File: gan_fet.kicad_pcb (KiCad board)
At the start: 2 copper layers, 13 x 22.2 mm, 6 parts, among them J1 Conn_01x04_Male, Q1 EPC2036, U1 NPC81074

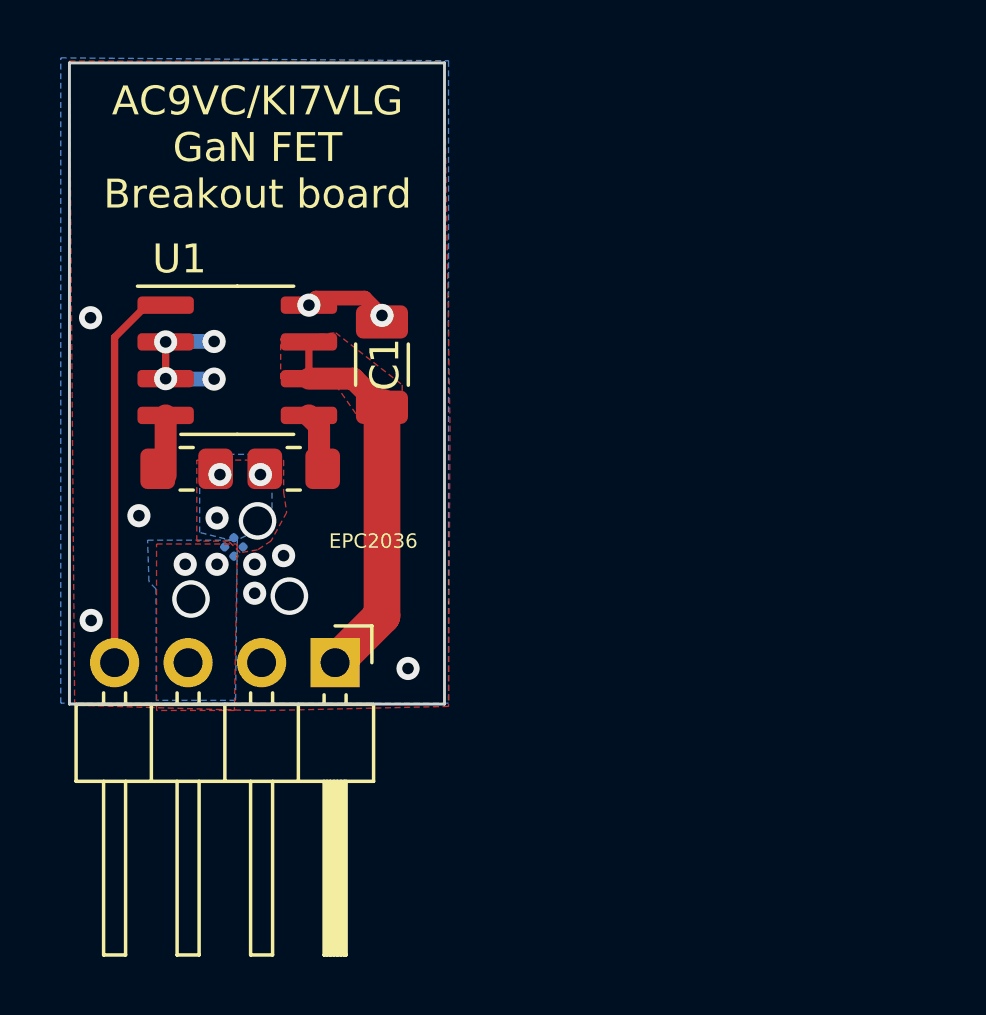
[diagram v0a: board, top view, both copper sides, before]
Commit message: rev_1 board
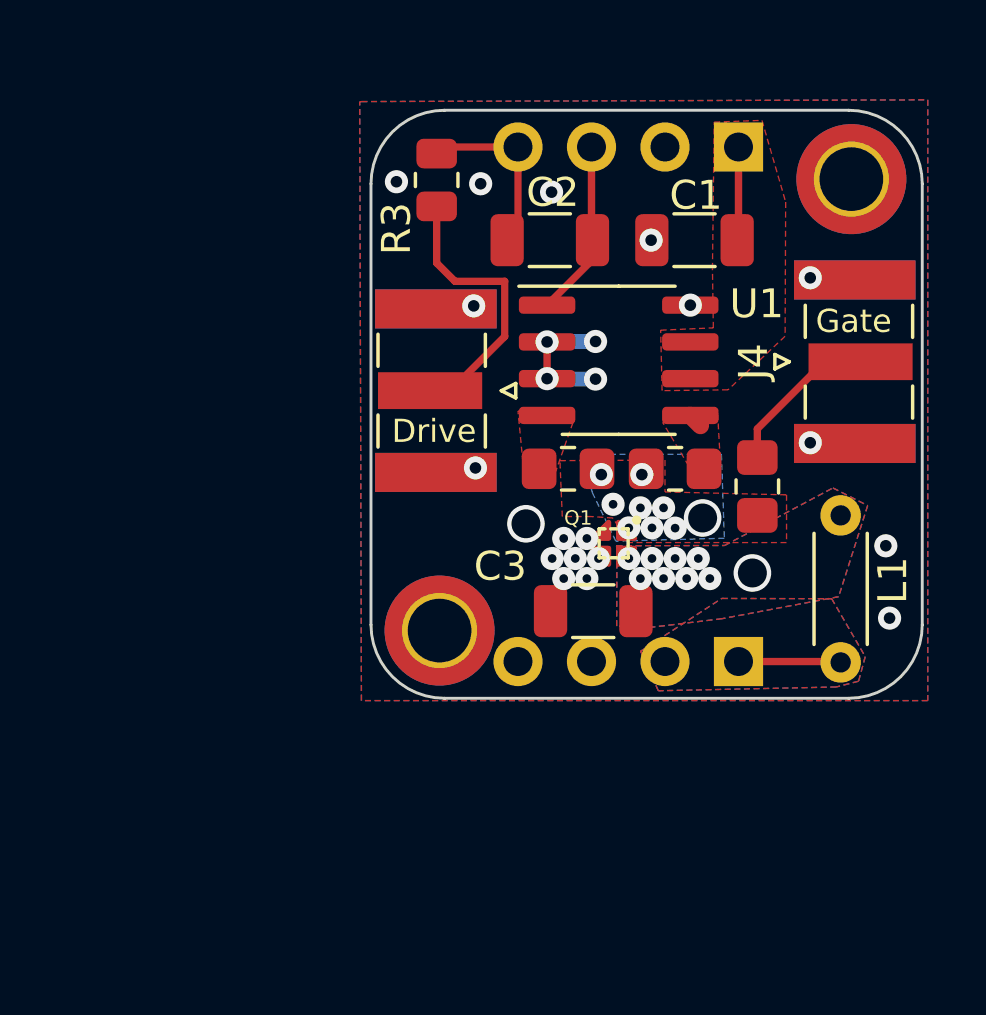
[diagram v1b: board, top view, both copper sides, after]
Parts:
- added C2: 100n, Capacitor_SMD:C_1206_3216Metric, F.Cu at (153.5, 84.5)
- added C3: 33p, Capacitor_SMD:C_1206_3216Metric, F.Cu at (155.0, 97.3)
- added J2: Driver TestPoint, Connector_Coaxial:SMA_Samtec_SMA-J-P-X-ST-EM1_EdgeMount, F.Cu at (149.6, 89.7)
- added J3: Conn_01x04_Male, Connector_PinHeader_2.54mm:PinHeader_1x04_P2.54mm_Vertical, B.Cu at (160.0, 99.1)
- added J4: FetGate test point, Connector_Coaxial:SMA_Samtec_SMA-J-P-X-ST-EM1_EdgeMount, F.Cu at (164.0, 88.7)
- added J5: Mounting Hole, MountingHole:MountingHole_2.2mm_M2_ISO14580_Pad_TopBottom, F.Cu at (163.9, 82.4)
- added J6: Conn_01x01_Male, MountingHole:MountingHole_2.2mm_M2_ISO14580_Pad_TopBottom, F.Cu at (149.7, 98.0)
- added L1: L, Resistor_THT:R_Axial_DIN0204_L3.6mm_D1.6mm_P5.08mm_Horizontal, F.Cu at (163.6, 99.1)
- added R3: 470, Resistor_SMD:R_0805_2012Metric, F.Cu at (149.6, 82.4)
- added R5: 470, Resistor_SMD:R_0805_2012Metric_Pad1.20x1.40mm_HandSolder, F.Cu at (160.7, 93.0)
- J1: footprint Connector_PinHeader_2.54mm:PinHeader_1x04_P2.54mm_Horizontal -> Connector_PinHeader_2.54mm:PinHeader_1x04_P2.54mm_Vertical; moved to B.Cu
- Q1: moved to F.Cu
- R1: value 1 -> 2.2
- R2: value 4.7 -> 2.2
- moved J1 22.6 mm to (160.0, 81.3), turned to 90 degrees
- moved R1 13.2 mm to (154.1, 92.4)
- moved R2 13.2 mm to (157.8, 92.4)
- moved U1 13.2 mm to (155.9, 88.7)
- moved Q1 12.5 mm to (155.7, 95.0), turned to -90 degrees
- moved C1 11.6 mm to (158.5, 84.5), turned to 180 degrees
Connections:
- J1 pad 3: /drain -> /driveBias
- Q1 pad 1: GND -> /fetGate
- Q1 pad 2: /drain -> GND
- Q1 pad 3: /fetGate -> Net-(C3-Pad1)
- Q1 pad 4: /drain -> GND
- U1 pad 1: /gate -> /driveBias
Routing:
- net +5V: track 14.0 -> 3.24 mm
- net Net-(J2-Pad1): track 0.00 -> 10.6 mm
- net /gate: track 12.8 -> 6.26 mm
- net /driveBias: track 0.00 -> 6.13 mm
- net Net-(J4-Pad1): track 0.00 -> 5.90 mm
- net /Vcc: track 0.00 -> 3.54 mm
- net GND: track 7.51 -> 4.63 mm, vias 14 -> 23
- net Net-(R2-Pad1): track 2.24 -> 0.49 mm
- net Net-(R1-Pad1): track 2.07 -> 0.39 mm
- net Net-(C3-Pad1): vias 0 -> 9
- net /fetGate: vias 4 -> 9
- net /drain: vias 3 -> 0
- added copper zone on B.Cu, net /Vcc
- added copper zone on F.Cu, net /Vcc
- added copper zone on B.Cu, net Net-(C3-Pad1)
- added copper zone on F.Cu, net Net-(C3-Pad1)
- added copper zone on F.Cu, net Net-(R1-Pad1)
- added copper zone on F.Cu, net Net-(R2-Pad1)
- removed copper zone on B.Cu, net /drain
- removed copper zone on F.Cu, net /drain
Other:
- board size 13 x 22.2 mm -> 19.1 x 20.3 mm
- rule pad_to_mask_clearance: 0 -> 0.0508
- board text added: "5V Gnd Bias Drive"
- board text added: "Drive"
- board text added: "GND"
- board text added: "Gate"
- board text added: "VCC"
- board text added: "rev_1"
- board text removed: "+5 S D G"
